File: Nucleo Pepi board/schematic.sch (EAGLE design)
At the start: 9 parts, among them J1 1X2-3.5MM

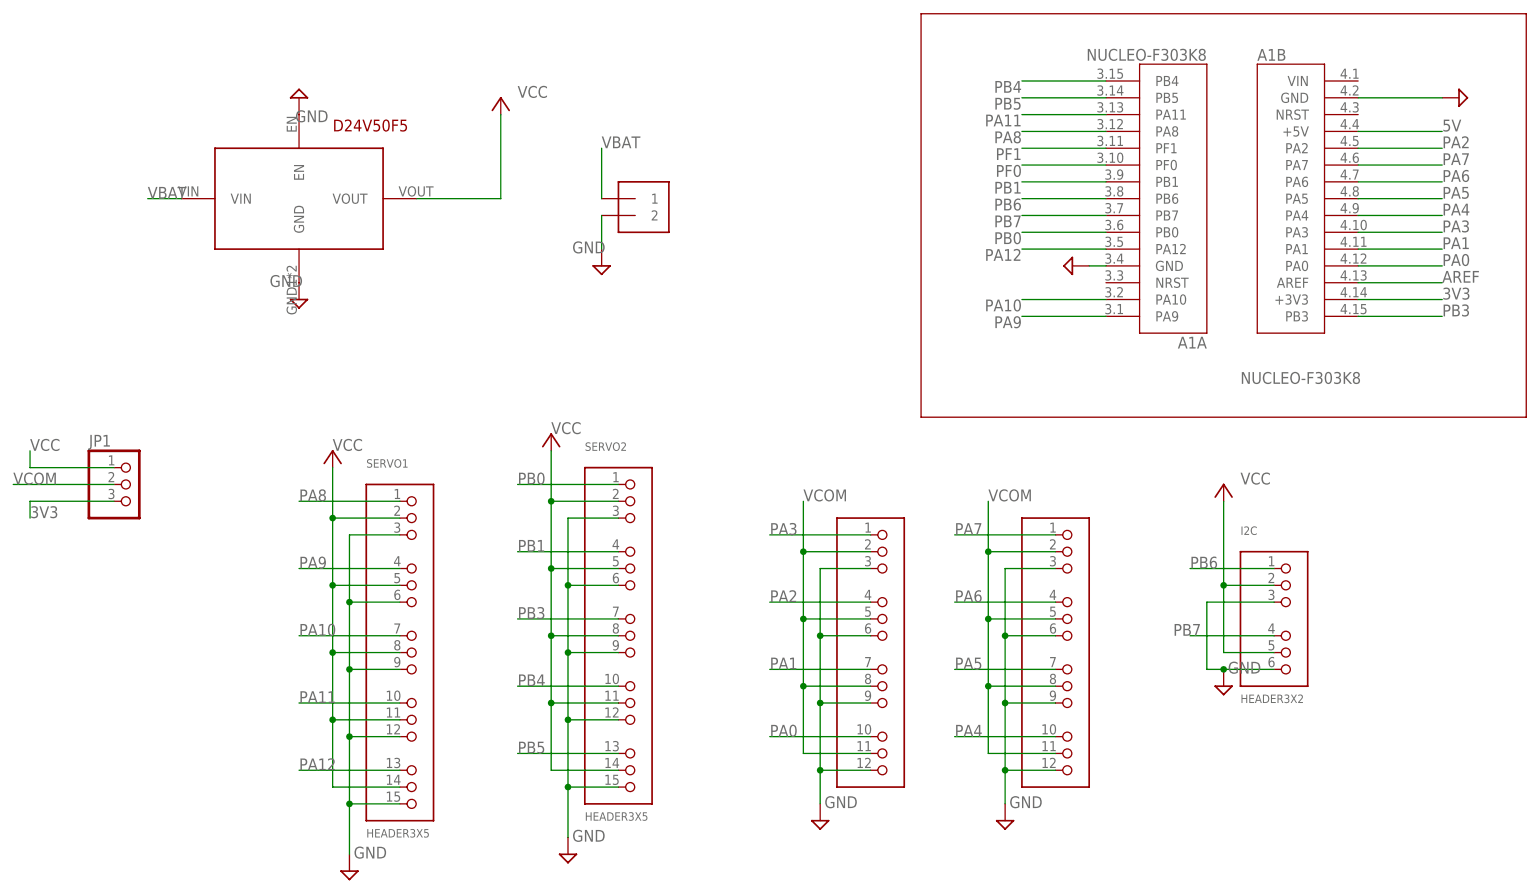
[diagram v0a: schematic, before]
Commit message: update
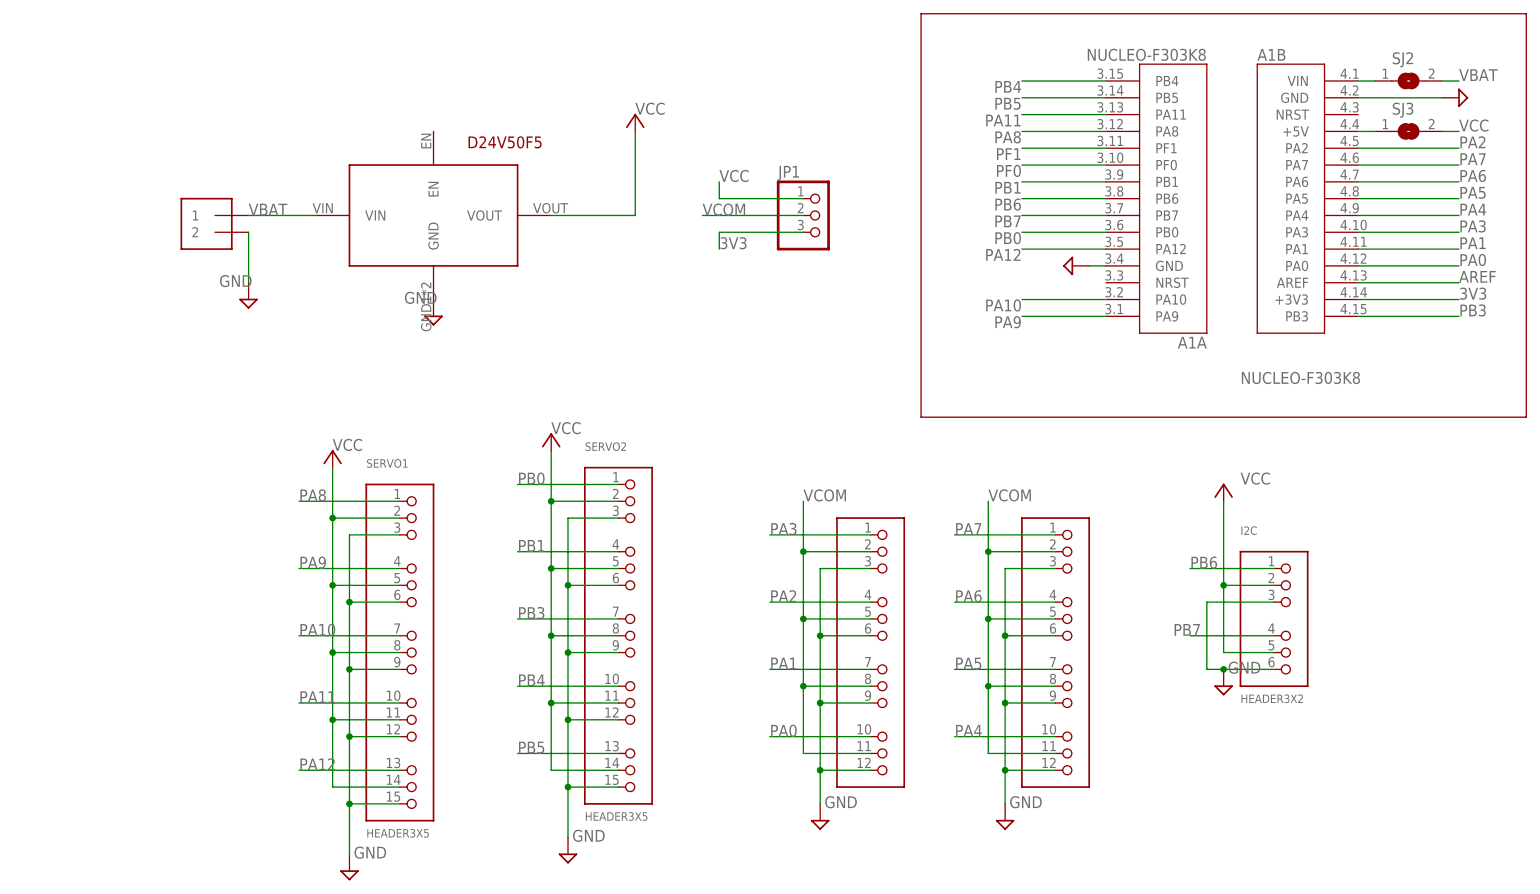
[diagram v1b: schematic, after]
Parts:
- added SJ2, SJ3: (no value), jumper:SJW
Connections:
- removed net 5V: A1B.+5V
- new net N$1: A1B.VIN, SJ2.1
- new net N$2: A1B.+5V, SJ3.1
- net GND: no longer U$1.EN
- net VBAT: now also SJ2.2
- net VCC: now also SJ3.2
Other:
- moved on the sheet: JP1
